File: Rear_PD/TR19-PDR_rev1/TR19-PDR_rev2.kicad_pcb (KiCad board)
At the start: 2 copper layers, 5 parts, among them J1 Conn_01x11_Female, J2 Conn_01x12_Female

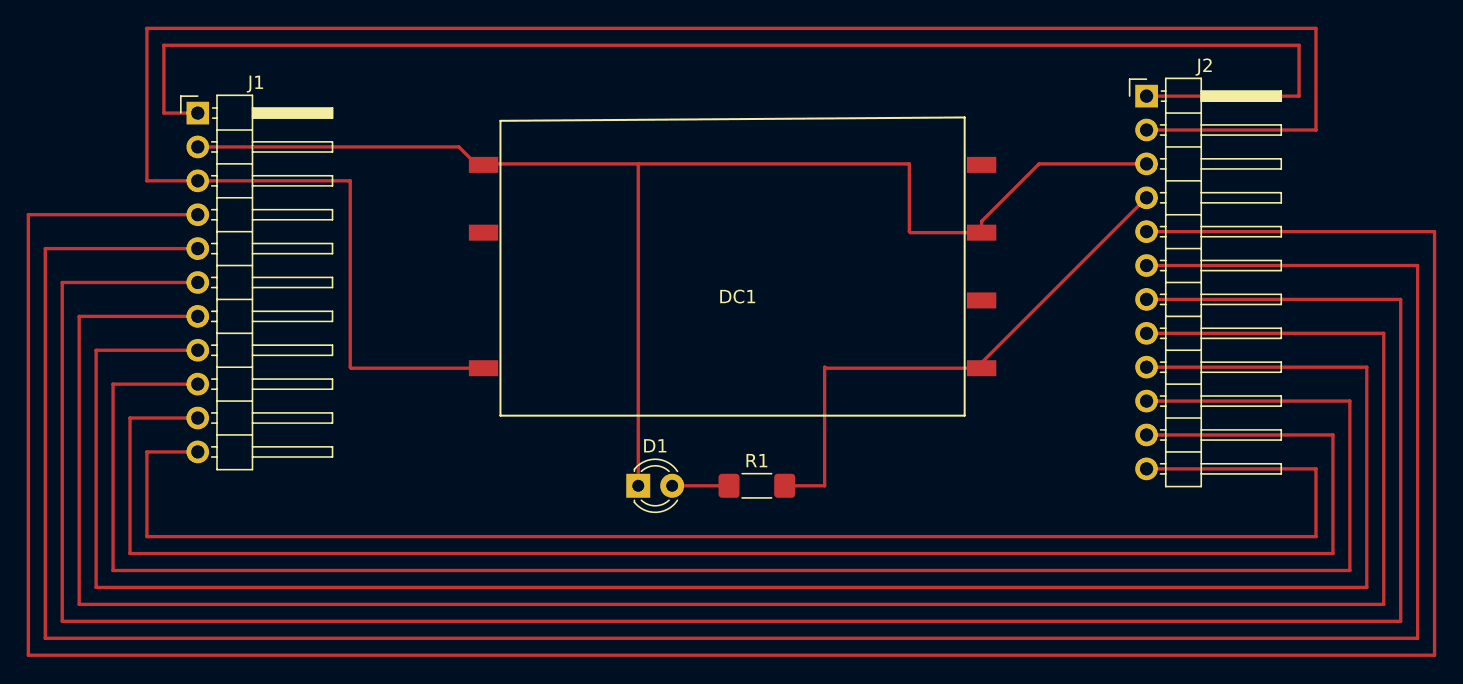
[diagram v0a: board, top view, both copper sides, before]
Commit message: PDB PCB Updates
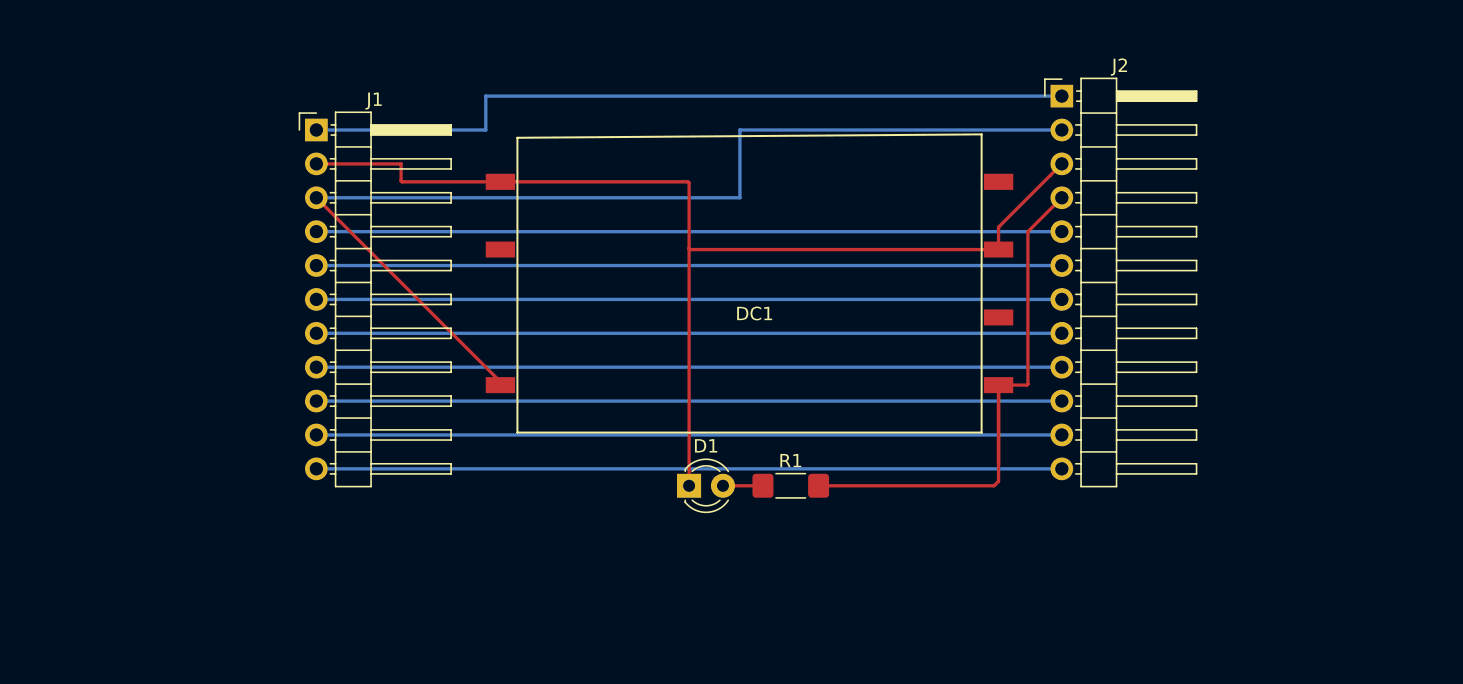
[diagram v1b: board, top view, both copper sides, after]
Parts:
- moved J1 8.98 mm to (101.6, 78.7)
- moved J2 6.35 mm to (157.5, 76.2)
- moved D1 3.81 mm to (129.5, 105.4)
- moved R1 2.54 mm to (137.2, 105.4)
- moved DC1 1.80 mm to (116.4, 101.7)
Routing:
- net Net-(J1-Pad4): track 204.5 -> 55.9 mm
- net Net-(J1-Pad5): track 191.8 -> 55.9 mm
- net Net-(J1-Pad6): track 179.1 -> 55.9 mm
- net Net-(J1-Pad7): track 166.4 -> 55.9 mm
- net Net-(J1-Pad8): track 153.7 -> 55.9 mm
- net Net-(J1-Pad9): track 141.0 -> 55.9 mm
- net Net-(DC1-Pad1): track 158.6 -> 80.7 mm
- net Net-(J1-Pad10): track 128.3 -> 55.9 mm
- net Net-(J1-Pad11): track 115.6 -> 55.9 mm
- net Net-(J1-Pad1): track 107.9 -> 58.4 mm
- net GND: track 103.6 -> 83.6 mm
- net Net-(DC1-Pad7): track 41.6 -> 44.0 mm
- net Net-(D1-Pad2): track 4.26 -> 2.99 mm
